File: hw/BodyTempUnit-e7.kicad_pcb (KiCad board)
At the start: 4 copper layers, 25 x 30 mm, 27 parts, among them IC1 MAX481CUA, IC2 MEGA8-MI, J1 CONN_IN, J2 CONN_OUT, U1 MAX30205MTA+21-0137I_T833-2-M, U2 LSM6DS3, U3 MCP1801T-3302I_OT

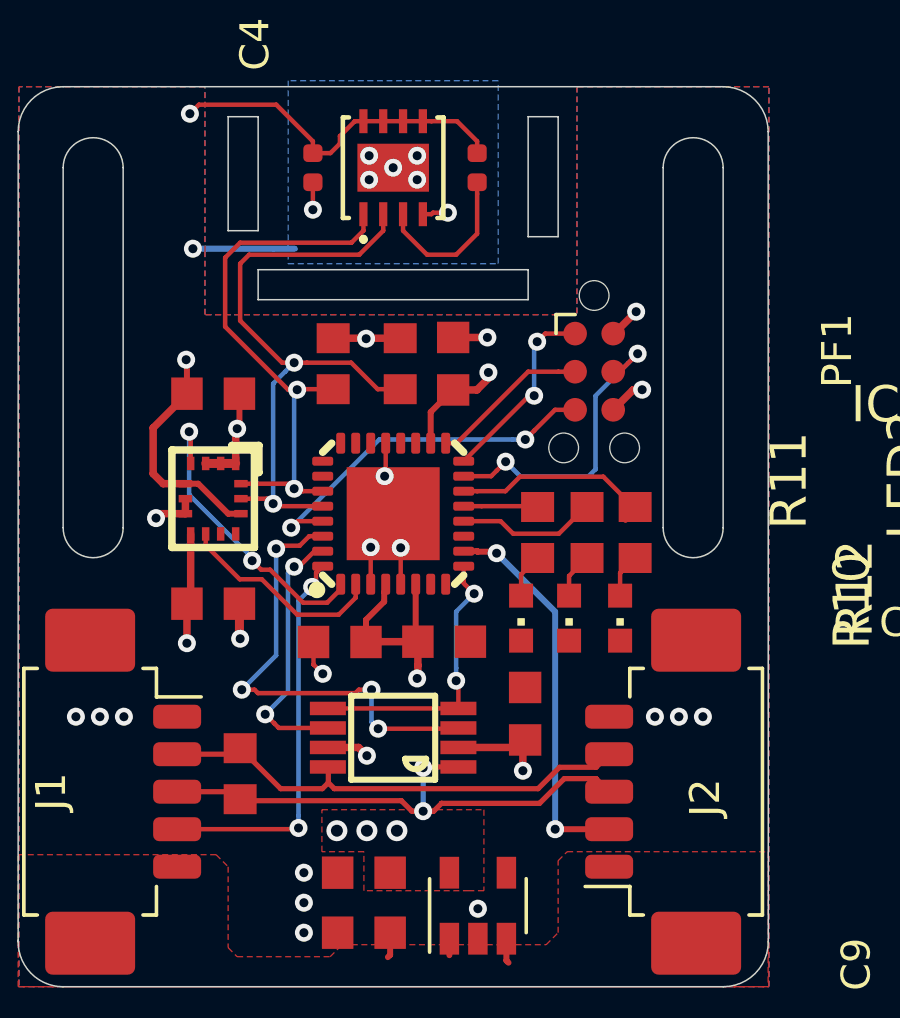
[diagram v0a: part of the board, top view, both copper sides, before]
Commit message: All routed, final check pending
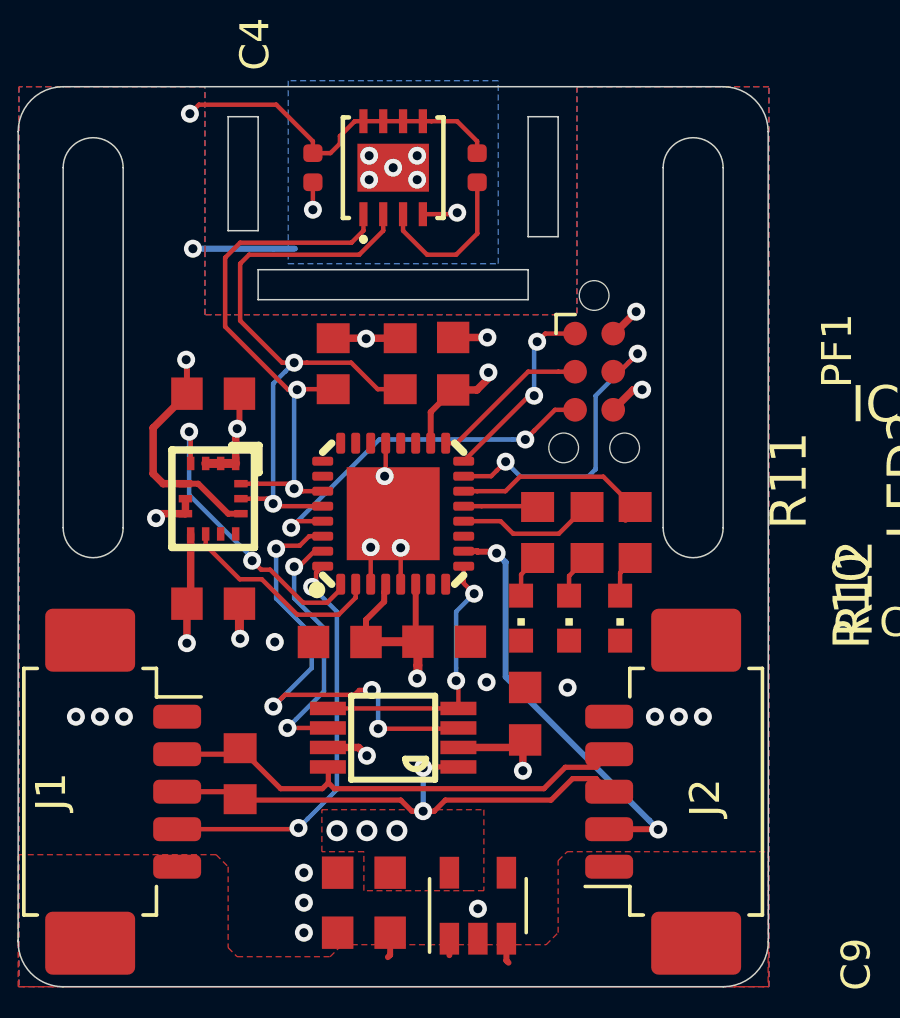
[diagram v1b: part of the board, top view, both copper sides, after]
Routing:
- net /SIG_OUT: track 12.9 -> 14.2 mm
- net GND: track 24.0 -> 23.1 mm, vias 28 -> 30
- net /SIG_IN: track 13.1 -> 13.8 mm

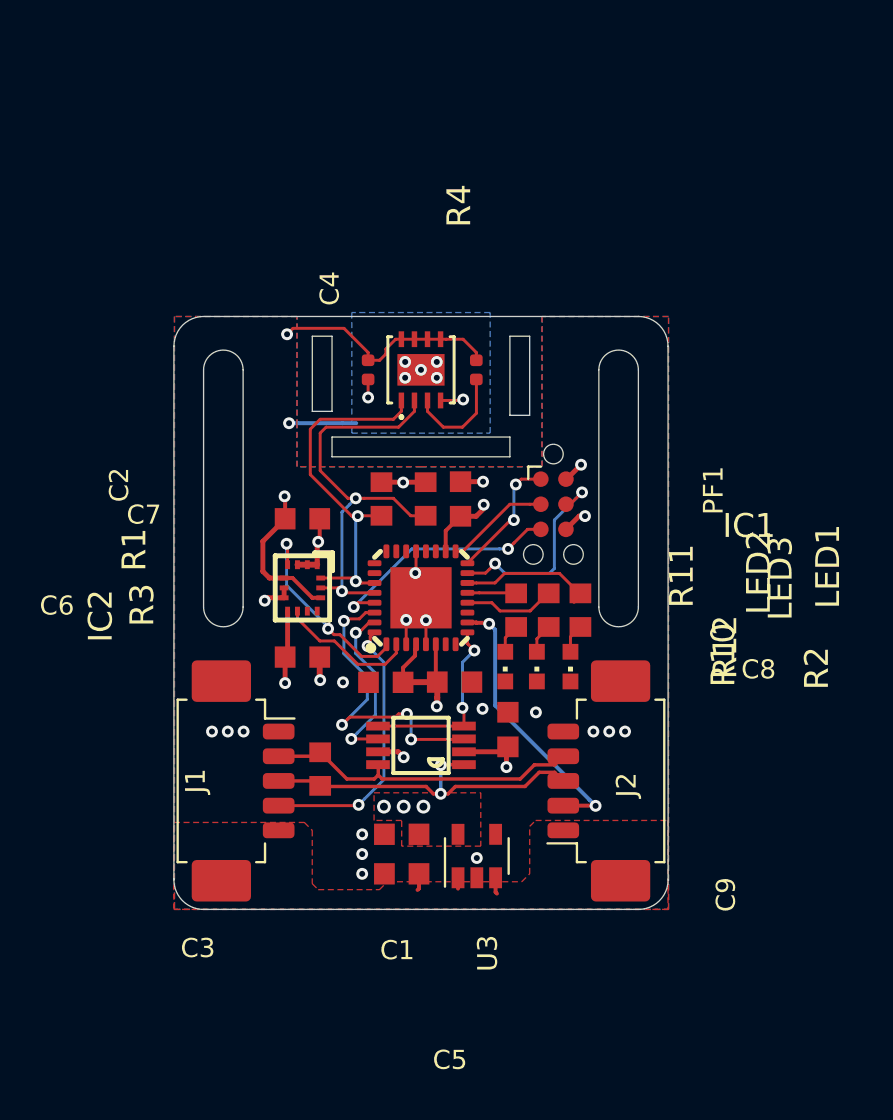
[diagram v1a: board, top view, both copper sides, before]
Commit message: version sent to production
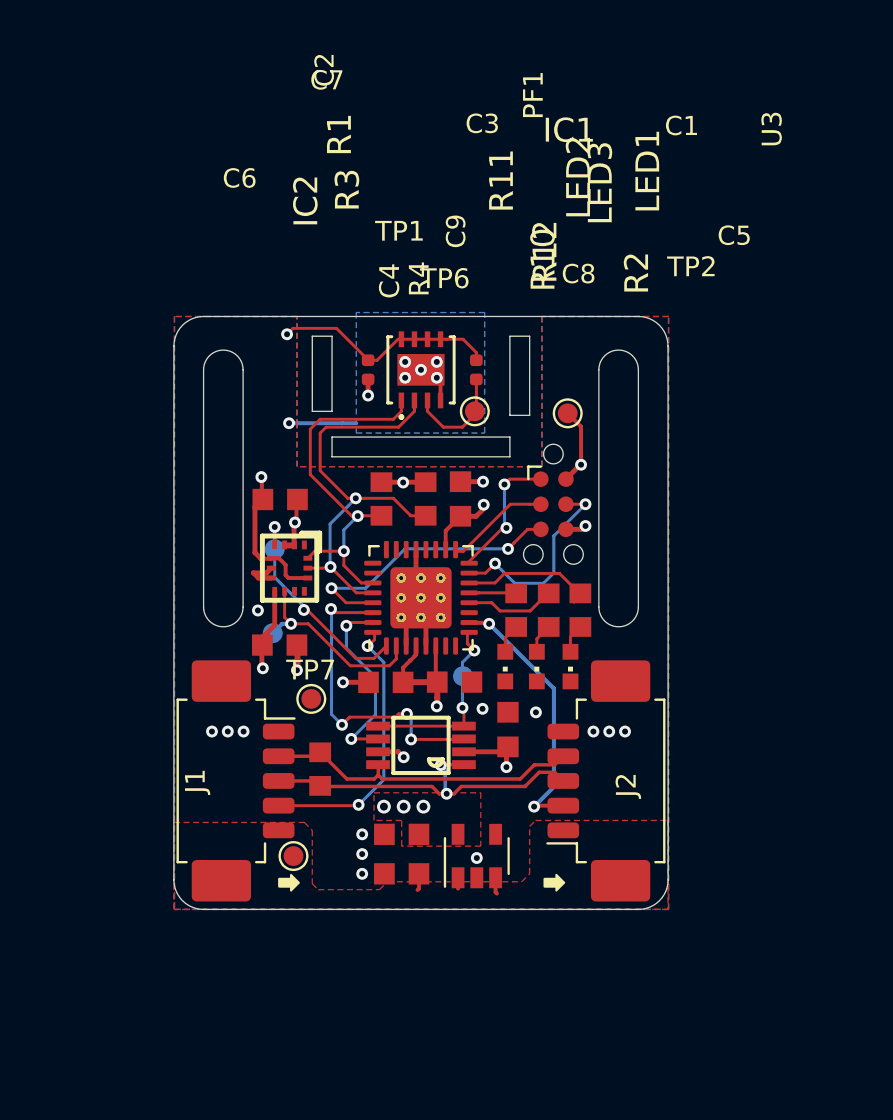
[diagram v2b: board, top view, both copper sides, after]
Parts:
- added G***: LOGO, logos:protospace, B.Cu at (69.8, 130.4)
- added TP1: TestPoint, TestPoint:TestPoint_Pad_D1.0mm, F.Cu at (71.0, 132.3)
- added TP2: TestPoint, TestPoint:TestPoint_Pad_D1.0mm, F.Cu at (84.9, 109.9)
- added TP3: TestPoint, TestPoint:TestPoint_Pad_D1.0mm, B.Cu at (79.6, 123.2)
- added TP4: TestPoint, TestPoint:TestPoint_Pad_D1.0mm, B.Cu at (70.1, 116.8)
- added TP5: TestPoint, TestPoint:TestPoint_Pad_D1.0mm, B.Cu at (70.0, 121.0)
- added TP6: TestPoint, TestPoint:TestPoint_Pad_D1.0mm, F.Cu at (80.2, 109.8)
- added TP7: TestPoint, TestPoint:TestPoint_Pad_D1.0mm, F.Cu at (72.0, 124.3)
- IC2: footprint BodyTempUnit-e7:MLF32 -> Package_DFN_QFN:QFN-32-1EP_5x5mm_P0.5mm_EP3.1x3.1mm_ThermalVias
- moved C7 1.49 mm to (70.4, 114.3)
- moved C6 1.30 mm to (70.3, 121.6)
- moved U2 1.19 mm to (70.9, 117.7)
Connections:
- IC2 pad 11: Net-(IC2-Pad11) -> (no net)
- IC2 pad 19: Net-(IC2-Pad19) -> (no net)
- IC2 pad 20: Net-(IC2-Pad20) -> (no net)
- IC2 pad 22: Net-(IC2-Pad22) -> (no net)
- IC2 pad 23: Net-(IC2-Pad23) -> (no net)
- IC2 pad 24: Net-(IC2-Pad24) -> (no net)
- IC2 pad 25: Net-(IC2-Pad25) -> (no net)
- IC2 pad 26: Net-(IC2-Pad26) -> (no net)
- IC2 pad 7: Net-(IC2-Pad7) -> (no net)
- IC2 pad 8: Net-(IC2-Pad8) -> (no net)
- U2 pad 10: Net-(U2-Pad10) -> (no net)
- U2 pad 11: Net-(U2-Pad11) -> (no net)
- U3 pad 4: Net-(U3-Pad4) -> (no net)
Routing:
- net /LSM_INT2: track 7.02 -> 10.00 mm, vias 0 -> 1
- net VCC: track 40.8 -> 43.3 mm
- net /RST: track 12.2 -> 14.3 mm
- net /LSM_INT1: track 10.1 -> 11.2 mm
- net /RS485_DI: track 8.81 -> 9.68 mm
- net GND: track 23.1 -> 23.9 mm, vias 30 -> 26
- net /SIG_OUT: track 14.2 -> 13.6 mm
- net /SDA: track 18.6 -> 19.1 mm
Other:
- board text added: "Body Sense Array V0.1"
- board text added: "~"
